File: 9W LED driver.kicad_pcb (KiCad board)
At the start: 2 copper layers, 51.4 x 21.7 mm, 28 parts, among them IC1 Si 9752 680PY89

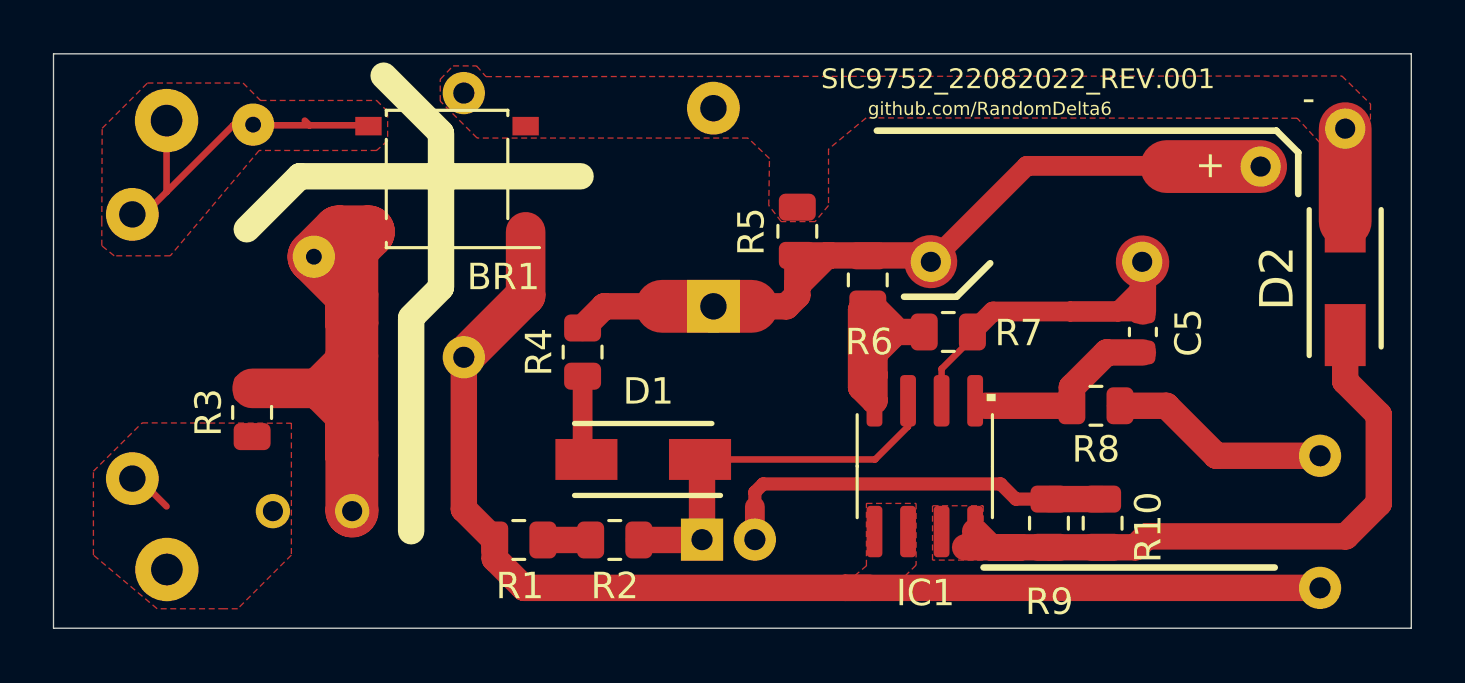
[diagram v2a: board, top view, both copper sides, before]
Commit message: Updated PCB Layout
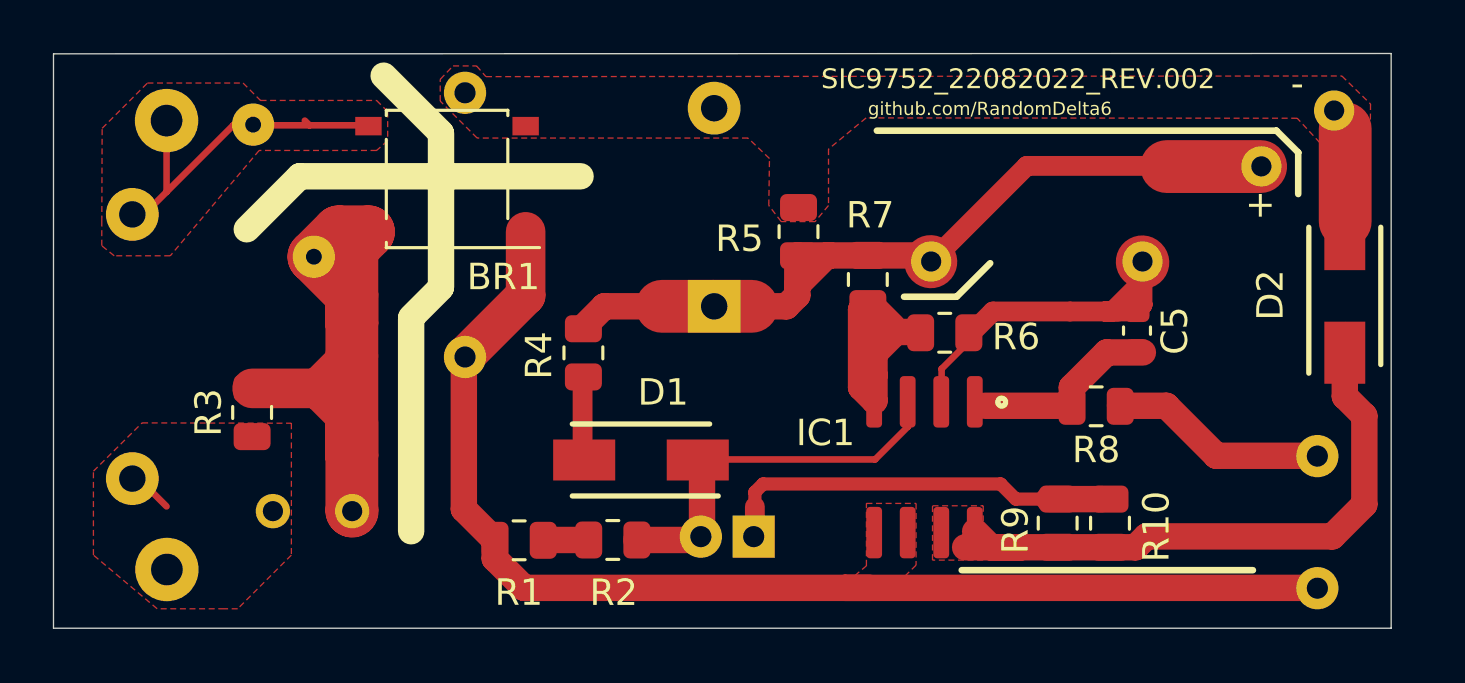
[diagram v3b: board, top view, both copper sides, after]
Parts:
- IC1: value Si 9752 680PY89 -> Sic9752
- moved C1 9.99 mm to (68.4, 62.3), turned to 90 degrees
- moved R7 3.64 mm to (83.7, 59.4), turned to 90 degrees
- moved R6 3.53 mm to (86.6, 61.4), turned to 0 degrees
- moved C3 1.96 mm to (79.4, 69.1), turned to 180 degrees
- moved - 0.80 mm to (101.3, 53.0)
- moved D2 0.67 mm to (101.7, 60.0)
- moved REF** 0.58 mm to (71.0, 68.1)
- moved R9 0.33 mm to (90.9, 68.6), turned to 90 degrees
- moved R10 0.28 mm to (92.9, 68.6), turned to 90 degrees
- moved C5 0.23 mm to (93.9, 61.3), turned to 270 degrees
- moved C6 0.10 mm to (100.7, 66.0)
- moved D1 0.09 mm to (75.1, 66.2)
- moved R2 0.07 mm to (74.0, 69.2)
- turned R5 to 90 degrees
- turned R4 to 270 degrees
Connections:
- + pad 1: Net-(C4-Pad2) -> +ve_output
- - pad 1: -ve_Rail -> GNDS
- BR1 pad 2: -ve_Rail -> GNDS
- C1 pad 1: -ve_Rail -> +ve_Rail
- C1 pad 2: +ve_Rail -> GNDS
- C4 pad 1: Net-(C4-Pad2) -> +ve_output
- C4 pad 2: -ve_Rail -> GNDS
- D1 pad 1: Net-(C3-Pad1) -> Net-(C3-Pad2)
- D2 pad 2: -ve_Rail -> GNDS
- IC1 pad 1: Net-(C5-Pad1) -> Net-(C5-Pad2)
- IC1 pad 2: Net-(C5-Pad2) -> Net-(C5-Pad1)
- IC1 pad 3: Net-(C3-Pad1) -> Net-(C3-Pad2)
- IC1 pad 4: Net-(IC1-Pad4) -> Net-(R6-Pad1)
- L2 pad 1: Net-(C4-Pad2) -> +ve_output
- L2 pad 2: Net-(C5-Pad2) -> Net-(C5-Pad1)
- R10 pad 1: Net-(C3-Pad2) -> Net-(D2-Pad1)
- R10 pad 2: Net-(D2-Pad1) -> Net-(C3-Pad1)
- R2 pad 2: Net-(C3-Pad1) -> Net-(C3-Pad2)
- R4 pad 1: Net-(D1-Pad2) -> +ve_output
- R4 pad 2: Net-(C4-Pad2) -> Net-(D1-Pad2)
- R5 pad 1: -ve_Rail -> +ve_output
- R5 pad 2: Net-(C4-Pad2) -> GNDS
- R6 pad 1: Net-(C4-Pad2) -> Net-(R6-Pad1)
- R6 pad 2: Net-(IC1-Pad4) -> Net-(C5-Pad1)
- R7 pad 1: Net-(IC1-Pad4) -> Net-(R6-Pad1)
- R7 pad 2: Net-(C5-Pad2) -> +ve_output
- R8 pad 2: Net-(C5-Pad1) -> Net-(C5-Pad2)
- R9 pad 1: Net-(C3-Pad2) -> Net-(D2-Pad1)
- R9 pad 2: Net-(D2-Pad1) -> Net-(C3-Pad1)
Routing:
- net Net-(C4-Pad2): track 31.1 -> 0.00 mm
- net +ve_output: track 0.00 -> 31.1 mm
- net Net-(R6-Pad1): track 0.00 -> 10.8 mm
- net Net-(IC1-Pad4): track 10.8 -> 0.00 mm
- net Net-(C5-Pad1): track 7.50 -> 15.1 mm
- net Net-(C5-Pad2): track 14.9 -> 7.50 mm
- net GNDS: track 0.00 -> 3.58 mm
- net -ve_Rail: track 3.58 -> 0.00 mm
- net Net-(C3-Pad2): track 15.9 -> 15.1 mm
- net Net-(C3-Pad1): track 15.1 -> 15.9 mm
- added copper zone on F.Cu, net GNDS
- removed copper zone on F.Cu, net -ve_Rail
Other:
- board size 51.4 x 21.7 mm -> 50.6 x 21.8 mm
- board text added: "SIC9752_22082022_REV.002"
- board text removed: "SIC9752_22082022_REV.001"
